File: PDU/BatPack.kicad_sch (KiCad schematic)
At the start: 1 part, among them J11 Screw_Terminal_01x02

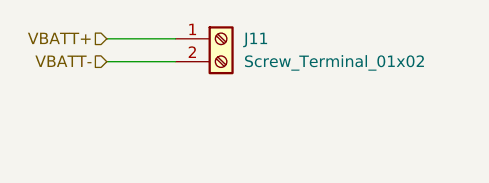
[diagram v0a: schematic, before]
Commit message: Last revision
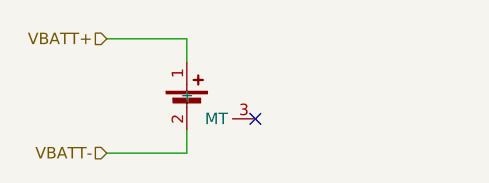
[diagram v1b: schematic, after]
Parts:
- removed J11: Screw_Terminal_01x02, symbol Connector:Screw_Terminal_01x02
- added M1: ~, Capstone:AA_Bat_Contact, symbol Capstone:BatPack
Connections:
- net VBATT+: now also M1.1 (+)
- net VBATT-: now also M1.2 (-)
- no-connect marks 0 -> 1
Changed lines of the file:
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@@
 		(comment 4 "Damien Huskic")
+	)
+	(no_connect
+		(at 167.64 97.79)
 	)
 	(wire
 		(pts
-			(xy 151.13 91.44) (xy 158.75 91.44)
+			(xy 160.02 101.6) (xy 160.02 99.06)
 		)
 		(stroke
@@
 	(wire
 		(pts
-			(xy 151.13 88.9) (xy 158.75 88.9)
+			(xy 151.13 101.6) (xy 160.02 101.6)
+		)
+		(stroke
+			(width 0)
+			(type default)
+		)
+	)
+	(wire
+		(pts
+			(xy 160.02 88.9) (xy 160.02 91.44)
+		)
+		(stroke
+			(width 0)
+			(type default)
+		)
+	)
+	(wire
+		(pts
+			(xy 151.13 88.9) (xy 160.02 88.9)
 		)
 		(stroke
@@
 	(hierarchical_label "VBATT-"
 		(shape input)
-		(at 151.13 91.44 180)
+		(at 151.13 101.6 180)
 		(fields_autoplaced yes)
 		(effects
@@
 	)
 	(symbol
-		(lib_id "Connector:Screw_Terminal_01x02")
-		(at 163.83 88.9 0)
+		(lib_id "Capstone:BatPack")
+		(at 160.02 95.25 0)
 		(unit 1)
 		(exclude_from_sim no)
@@
 		(dnp no)
 		(fields_autoplaced yes)
-		(property "Reference" "J11"
-			(at 166.37 88.8999 0)
+		(property "Reference" "M1"
+			(at 156.21 94.6784 0)
 			(effects
 				(font
 					(size 1.27 1.27)
 				)
-				(justify left)
+				(justify right)
+				(hide yes)
 			)
 		)
-		(property "Value" "Screw_Terminal_01x02"
-			(at 166.37 91.4399 0)
+		(property "Value" "~"
+			(at 156.21 96.5835 0)
 			(effects
 				(font
 					(size 1.27 1.27)
 				)
-				(justify left)
+				(justify right)
 			)
 		)
-		(property "Footprint" ""
-			(at 163.83 88.9 0)
+		(property "Footprint" "Capstone:AA_Bat_Contact"
+			(at 156.21 95.25 0)
 			(effects
 				(font
@@
 			)
 		)
-		(property "Datasheet" "~"
-			(at 163.83 88.9 0)
+		(property "Datasheet" ""
+			(at 156.21 95.25 0)
 			(effects
 				(font
@@
 			)
 		)
-		(property "Description" "Generic screw terminal, single row, 01x02, script generated (kicad-library-utils/schlib/autogen/connector/)"
-			(at 163.83 88.9 0)
+		(property "Description" ""
+			(at 156.21 95.25 0)
 			(effects
 				(font
@@
 			)
 		)
+		(pin "2"
+		)
 		(pin "1"
 		)
-		(pin "2"
+		(pin "3"
 		)
 		(instances
 			(project ""
 				(path "/365e279d-a26e-42dd-bfe1-7a86883567c0/afd244f8-33c3-4733-97b0-c9d5fe47b0fd"
-					(reference "J11")
+					(reference "M1")
 					(unit 1)
 				)
